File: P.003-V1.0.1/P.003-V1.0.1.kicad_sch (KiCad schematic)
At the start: 0 parts

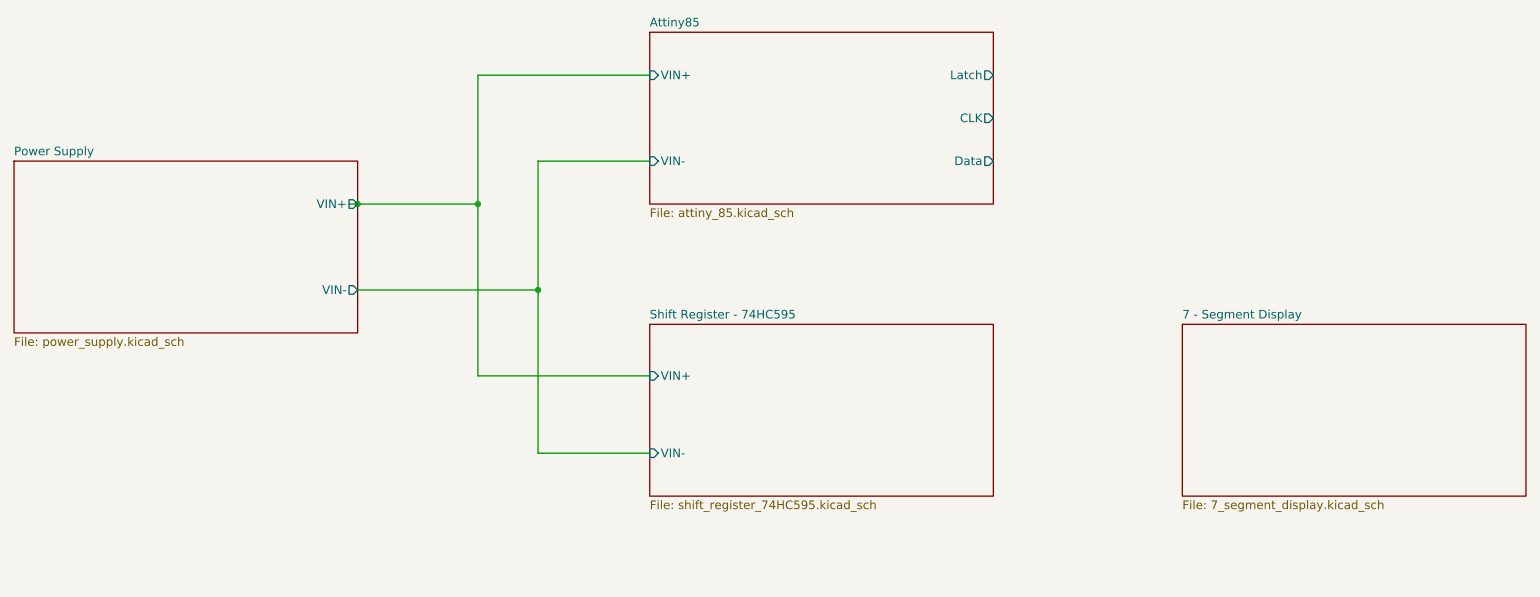
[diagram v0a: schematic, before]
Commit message: Schematic wired
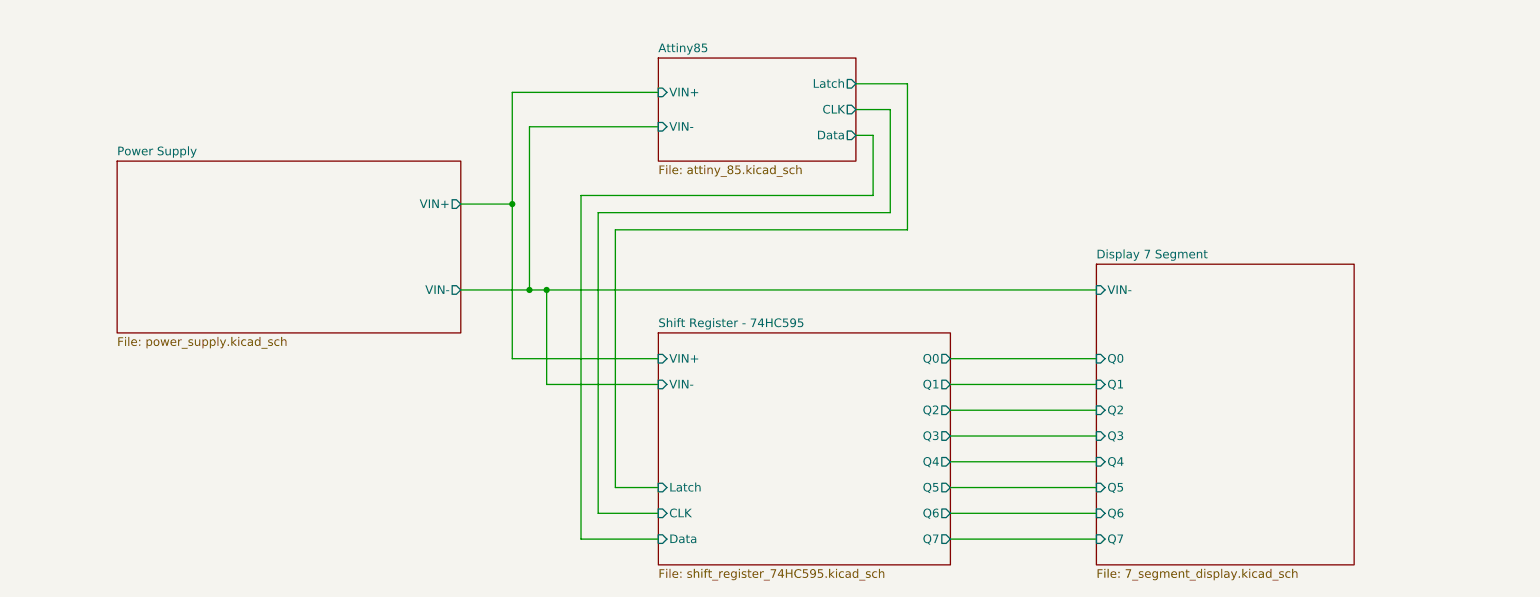
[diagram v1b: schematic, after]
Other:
- sheet 7 - Segment Display renamed Display 7 Segment
- sheet Display 7 Segment ports: added Q0, Q1, Q2, Q3, Q4, Q5, Q6, Q7, VIN-; removed none
- sheet Shift Register - 74HC595 ports: added CLK, Data, Latch, Q0, Q1, Q2, Q3, Q4, Q5, Q6, Q7; removed none
- company: (none) -> GSAS - Labs
- title: (none) -> Electronic Dice
